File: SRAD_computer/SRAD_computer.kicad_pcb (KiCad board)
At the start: 2 copper layers, 56 parts, among them J1 Terminal_3, J2 Conn_01x02, J3 UJ20-C-H-G-SMT-1-P16-TR, J4 Terminal_2, Q1 MMBT5551L, Q3 FDN340P, U1 NCP1117-3.3_SOT223, U2 W25Q128JVS, U3 RP2040, U4 BME280, U5 MPU-9250, U6 SAM-M8Q-0-10, Y1 ABM8-272-T3

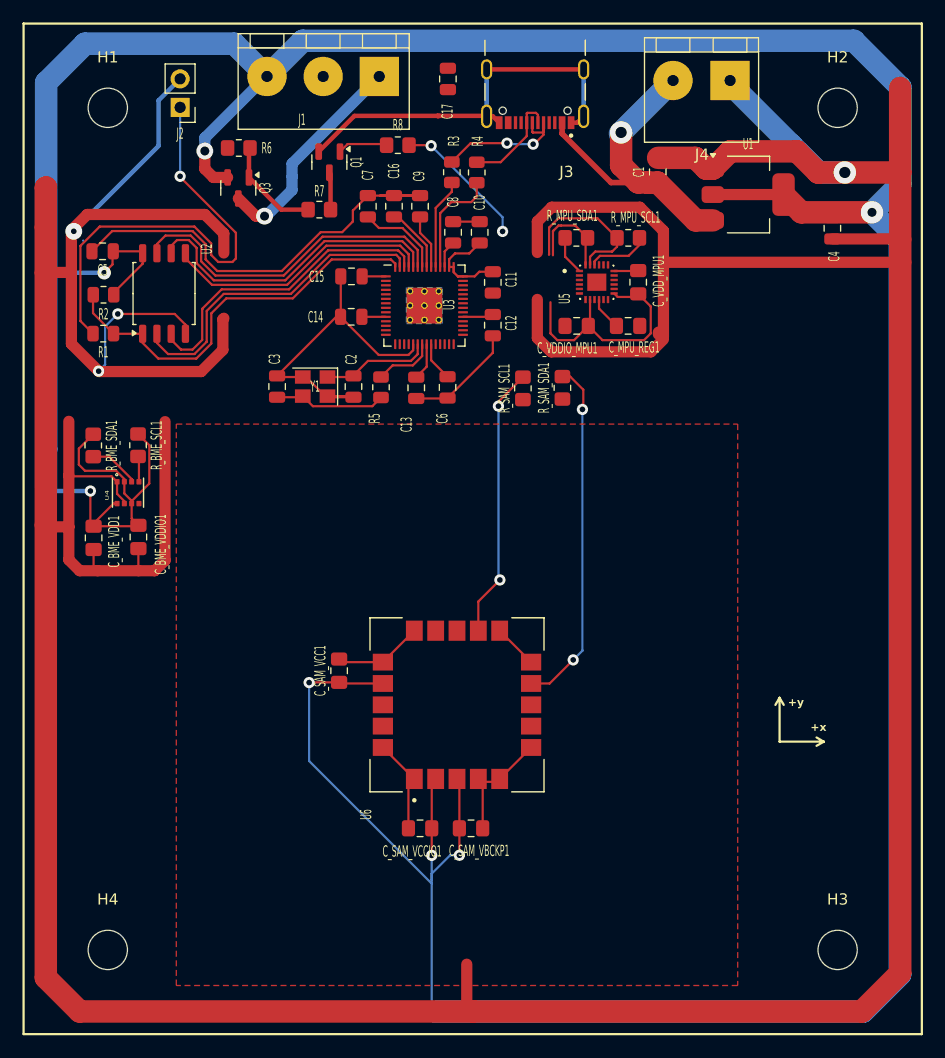
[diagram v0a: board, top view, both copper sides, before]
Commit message: PCB v1
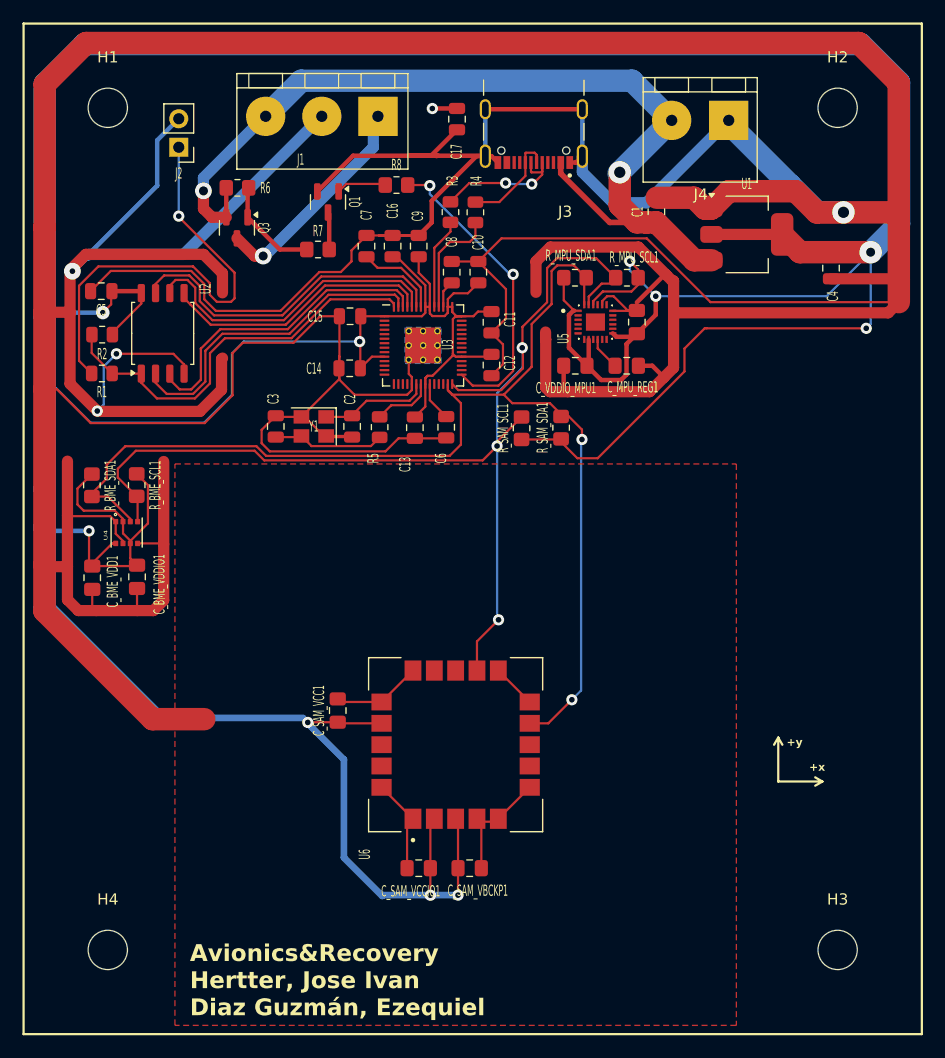
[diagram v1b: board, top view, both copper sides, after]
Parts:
- moved C14 4.59 mm to (79.0, 80.7)
- moved C17 3.67 mm to (88.6, 58.5)
- moved C11 3.55 mm to (91.7, 76.6)
- moved C12 3.55 mm to (91.7, 80.4)
- moved C3 3.55 mm to (72.5, 85.9)
- moved C_BME_VDDIO1 3.55 mm to (60.1, 99.3)
- moved C_MPU_REG1 3.55 mm to (103.7, 80.5)
- moved R_MPU_SDA1 3.55 mm to (99.1, 72.6)
- moved C13 3.55 mm to (84.8, 86.0)
- moved C15 3.55 mm to (79.1, 76.1)
- moved C16 3.55 mm to (82.9, 69.8)
- moved C2 3.55 mm to (79.3, 85.9)
- moved C7 3.55 mm to (80.5, 69.8)
- moved C9 3.55 mm to (85.2, 69.8)
- moved C_BME_VDD1 3.55 mm to (56.1, 99.4)
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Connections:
- J1 pad 3: +3V3 -> VBUS
- Q3 pad 2: +3V3 -> VBUS
- R6 pad 1: +3V3 -> VBUS
- R8 pad 1: /power_cam -> /GPIO18
- R_BME_SCL1 pad 2: /SCL -> /GPIO17
- R_BME_SDA1 pad 2: /SDA -> /GPIO16
- R_MPU_SCL1 pad 2: /SCL -> /GPIO17
- R_MPU_SDA1 pad 2: /SDA -> /GPIO16
- R_SAM_SCL1 pad 2: /SCL -> /GPIO17
- R_SAM_SDA1 pad 2: /SDA -> /GPIO16
- U4 pad 3: /SDA -> /GPIO16
- U4 pad 4: /SCL -> /GPIO17
- U4 pad 5: unconnected-(U4-SDO-Pad5) -> GND
- U5 pad 23: /SCL -> /GPIO17
- U5 pad 24: /SDA -> /GPIO16
- U6 pad 12: /SCL -> /GPIO17
- U6 pad 9: /SDA -> /GPIO16
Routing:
- net /GPIO16: track 0.00 -> 108.2 mm, vias 0 -> 2
- net GND: track 613.1 -> 720.4 mm
- net /GPIO17: track 0.00 -> 103.2 mm, vias 0 -> 3
- net VBUS: track 31.1 -> 85.6 mm, vias 1 -> 2
- net /SDA: track 44.3 -> 0.00 mm, vias 2 -> 0
- net /SCL: track 40.4 -> 0.00 mm, vias 2 -> 0
- net /GPIO18: track 0.00 -> 27.6 mm, vias 0 -> 2
- net /power_cam: track 12.3 -> 0.00 mm, vias 2 -> 0
- net +3V3: track 462.4 -> 470.2 mm, vias 7 -> 11
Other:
- board text added: "Avionics&Recovery Hertter, Jose Ivan Diaz Guzmán, Ezequiel"
